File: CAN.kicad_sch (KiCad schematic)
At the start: 15 parts, among them U17 ADM3055E, U18 CDSOT23-T24CAN

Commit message: added more part numbers
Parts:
- R34: P/N (none) -> CRCW08050000Z0EAC
- R35: P/N (none) -> CRCW080559R0FKEA
- U17: Mouser Part Number (none) -> 584-ADM3055EBRIZ; P/N (none) -> ADM3055EBRIZ
- U18: Mouser Part Number (none) -> 652-CDSOT23-T24CAN
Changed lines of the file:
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@@
       (effects (font (size 1.27 1.27)) hide)
     )
-    (property "Datasheet" "" (at 204.47 83.82 0)
+    (property "Datasheet" "https://www.vishay.com/docs/20035/dcrcwe3.pdf" (at 204.47 83.82 0)
       (effects (font (size 1.27 1.27)) hide)
     )
     (property "Mouser Part Number" "71-CRCW080559R0FKEA" (at 204.47 83.82 0)
+      (effects (font (size 1.27 1.27)) hide)
+    )
+    (property "P/N" "CRCW080559R0FKEA" (at 204.47 83.82 0)
       (effects (font (size 1.27 1.27)) hide)
     )
@@
     (property "Datasheet" "https://www.mouser.com/datasheet/2/609/ADM3055E-3057E-1509677.pdf" (at 111.76 82.55 0)
       (effects (font (size 1.524 1.524)) hide)
+    )
+    (property "Mouser Part Number" "584-ADM3055EBRIZ" (at 111.76 85.09 0)
+      (effects (font (size 1.27 1.27)) hide)
+    )
+    (property "P/N" "ADM3055EBRIZ" (at 111.76 85.09 0)
+      (effects (font (size 1.27 1.27)) hide)
     )
     (pin "1")
@@
       (effects (font (size 1.524 1.524)) hide)
     )
-    (property "Mouser Part Number" "" (at 207.01 66.04 0)
+    (property "Mouser Part Number" "652-CDSOT23-T24CAN" (at 207.01 66.04 0)
       (effects (font (size 1.27 1.27)) hide)
     )
@@
       (effects (font (size 1.27 1.27)) hide)
     )
-    (property "Datasheet" "" (at 142.24 99.06 0)
+    (property "Datasheet" "https://www.vishay.com/docs/28773/crcwce3.pdf" (at 142.24 99.06 0)
       (effects (font (size 1.27 1.27)) hide)
     )
@@
       (effects (font (size 1.27 1.27)) hide)
     )
+    (property "P/N" "CRCW08050000Z0EAC" (at 142.24 99.06 0)
+      (effects (font (size 1.27 1.27)) hide)
+    )

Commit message: added part numbers
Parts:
- C33, C38: P/N (none) -> 0805YC106KAT2A
- C34, C35, C39: Mouser Part Number 80-C0805C104K3R -> 80-C0805C104M5R; P/N (none) -> C0805C104M5RACTU
- C36: Mouser Part Number 80-C0805X103K1R3316 -> 80-C0805C104M5R; P/N (none) -> C0805C104M5RACTU
- C37: Mouser Part Number 80-C0805C224J1RECTU -> 80-C0805C224K5R; P/N (none) -> C0805C224K5RACTU
- C40: Mouser Part Number 80-C0805X103K1R3316 -> 80-C0805C103J5R; P/N (none) -> C0805C103J5RACTU
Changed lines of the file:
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@@
       (effects (font (size 1.27 1.27)) hide)
     )
-    (property "Datasheet" "~" (at 74.93 78.74 0)
-      (effects (font (size 1.27 1.27)) hide)
-    )
-    (property "Mouser Part Number" "80-C0805X103K1R3316 " (at 74.93 78.74 0)
+    (property "Datasheet" "https://www.mouser.com/datasheet/2/212/KEM_C1002_X7R_SMD-1102033.pdf" (at 74.93 78.74 0)
+      (effects (font (size 1.27 1.27)) hide)
+    )
+    (property "Mouser Part Number" "80-C0805C104M5R" (at 74.93 78.74 0)
+      (effects (font (size 1.27 1.27)) hide)
+    )
+    (property "P/N" "C0805C104M5RACTU" (at 74.93 78.74 0)
       (effects (font (size 1.27 1.27)) hide)
     )
@@
       (effects (font (size 1.27 1.27)) hide)
     )
-    (property "Datasheet" "~" (at 175.26 74.93 0)
-      (effects (font (size 1.27 1.27)) hide)
-    )
-    (property "Mouser Part Number" "80-C0805X103K1R3316 " (at 175.26 74.93 0)
+    (property "Datasheet" "https://www.mouser.com/datasheet/2/212/KEM_C1002_X7R_SMD-1102033.pdf" (at 175.26 74.93 0)
+      (effects (font (size 1.27 1.27)) hide)
+    )
+    (property "Mouser Part Number" "80-C0805C103J5R" (at 175.26 74.93 0)
+      (effects (font (size 1.27 1.27)) hide)
+    )
+    (property "P/N" "C0805C103J5RACTU" (at 175.26 74.93 0)
       (effects (font (size 1.27 1.27)) hide)
     )
@@
       (effects (font (size 1.27 1.27)) hide)
     )
-    (property "Datasheet" "~" (at 57.785 78.74 0)
-      (effects (font (size 1.27 1.27)) hide)
-    )
-    (property "Mouser Part Number" "80-C0805C104K3R " (at 57.785 78.74 0)
+    (property "Datasheet" "https://www.mouser.com/datasheet/2/212/KEM_C1002_X7R_SMD-1102033.pdf" (at 57.785 78.74 0)
+      (effects (font (size 1.27 1.27)) hide)
+    )
+    (property "Mouser Part Number" "80-C0805C104M5R" (at 57.785 78.74 0)
+      (effects (font (size 1.27 1.27)) hide)
+    )
+    (property "P/N" "C0805C104M5RACTU" (at 57.785 78.74 0)
       (effects (font (size 1.27 1.27)) hide)
     )
@@
       (effects (font (size 1.27 1.27)) hide)
     )
-    (property "Datasheet" "~" (at 167.64 74.93 0)
-      (effects (font (size 1.27 1.27)) hide)
-    )
-    (property "Mouser Part Number" "80-C0805C104K3R " (at 167.64 74.93 0)
+    (property "Datasheet" "https://www.mouser.com/datasheet/2/212/KEM_C1002_X7R_SMD-1102033.pdf" (at 167.64 74.93 0)
+      (effects (font (size 1.27 1.27)) hide)
+    )
+    (property "Mouser Part Number" "80-C0805C104M5R" (at 167.64 74.93 0)
+      (effects (font (size 1.27 1.27)) hide)
+    )
+    (property "P/N" "C0805C104M5RACTU" (at 167.64 74.93 0)
       (effects (font (size 1.27 1.27)) hide)
     )
@@
       (effects (font (size 1.27 1.27)) hide)
     )
-    (property "Datasheet" "" (at 147.32 74.93 0)
-      (effects (font (size 1.27 1.27)) hide)
-    )
-    (property "Mouser Part Number" "80-C0805C224J1RECTU " (at 147.32 74.93 0)
+    (property "Datasheet" "https://www.mouser.com/datasheet/2/212/KEM_C1002_X7R_SMD-1102033.pdf" (at 147.32 74.93 0)
+      (effects (font (size 1.27 1.27)) hide)
+    )
+    (property "Mouser Part Number" "80-C0805C224K5R" (at 147.32 74.93 0)
+      (effects (font (size 1.27 1.27)) hide)
+    )
+    (property "P/N" "C0805C224K5RACTU" (at 147.32 74.93 0)
       (effects (font (size 1.27 1.27)) hide)
     )
@@
       (effects (font (size 1.27 1.27)) hide)
     )
-    (property "Datasheet" "~" (at 69.215 78.74 0)
-      (effects (font (size 1.27 1.27)) hide)
-    )
-    (property "Mouser Part Number" "80-C0805C104K3R " (at 69.215 78.74 0)
+    (property "Datasheet" "https://www.mouser.com/datasheet/2/212/KEM_C1002_X7R_SMD-1102033.pdf" (at 69.215 78.74 0)
+      (effects (font (size 1.27 1.27)) hide)
+    )
+    (property "Mouser Part Number" "80-C0805C104M5R" (at 69.215 78.74 0)
+      (effects (font (size 1.27 1.27)) hide)
+    )
+    (property "P/N" "C0805C104M5RACTU" (at 69.215 78.74 0)
       (effects (font (size 1.27 1.27)) hide)
     )
@@
     )
     (property "Mouser Part Number" "80-C0805C106K8RAUTO " (at 157.48 74.93 0)
+      (effects (font (size 1.27 1.27)) hide)
+    )
+    (property "P/N" "0805YC106KAT2A" (at 157.48 74.93 0)
       (effects (font (size 1.27 1.27)) hide)
     )
@@
       (effects (font (size 1.27 1.27)) hide)
     )
+    (property "P/N" "0805YC106KAT2A" (at 48.895 78.74 0)
+      (effects (font (size 1.27 1.27)) hide)
+    )

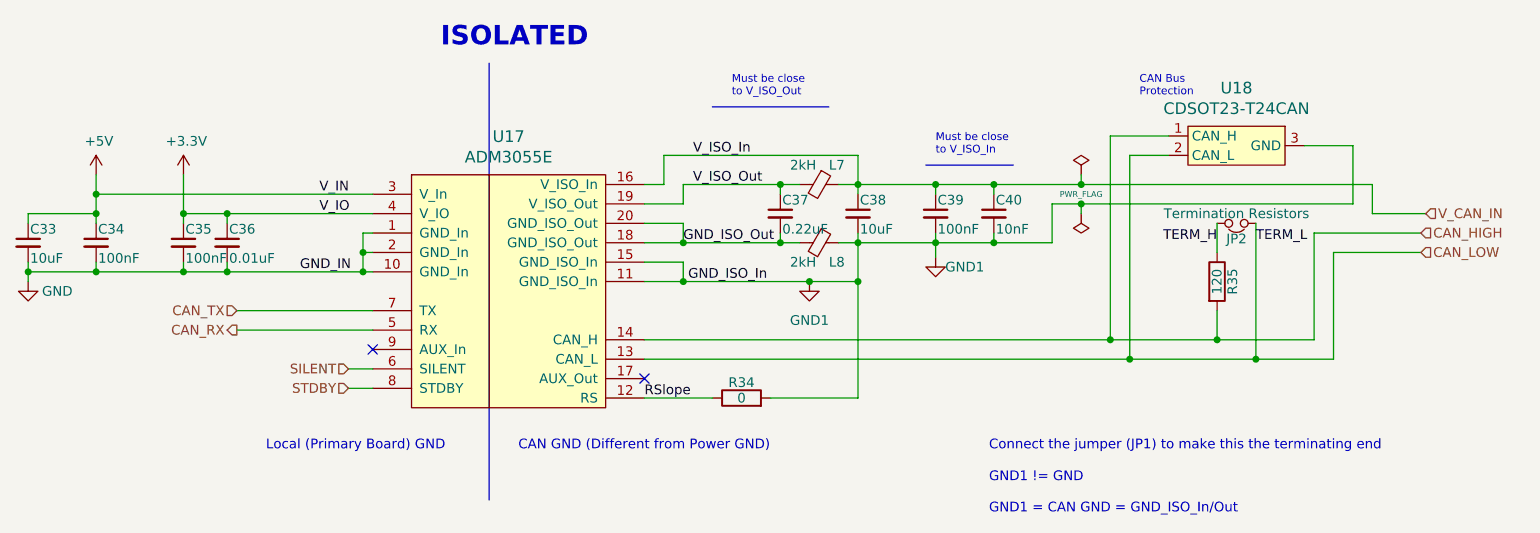
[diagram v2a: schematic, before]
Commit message: v1.2 initial changes
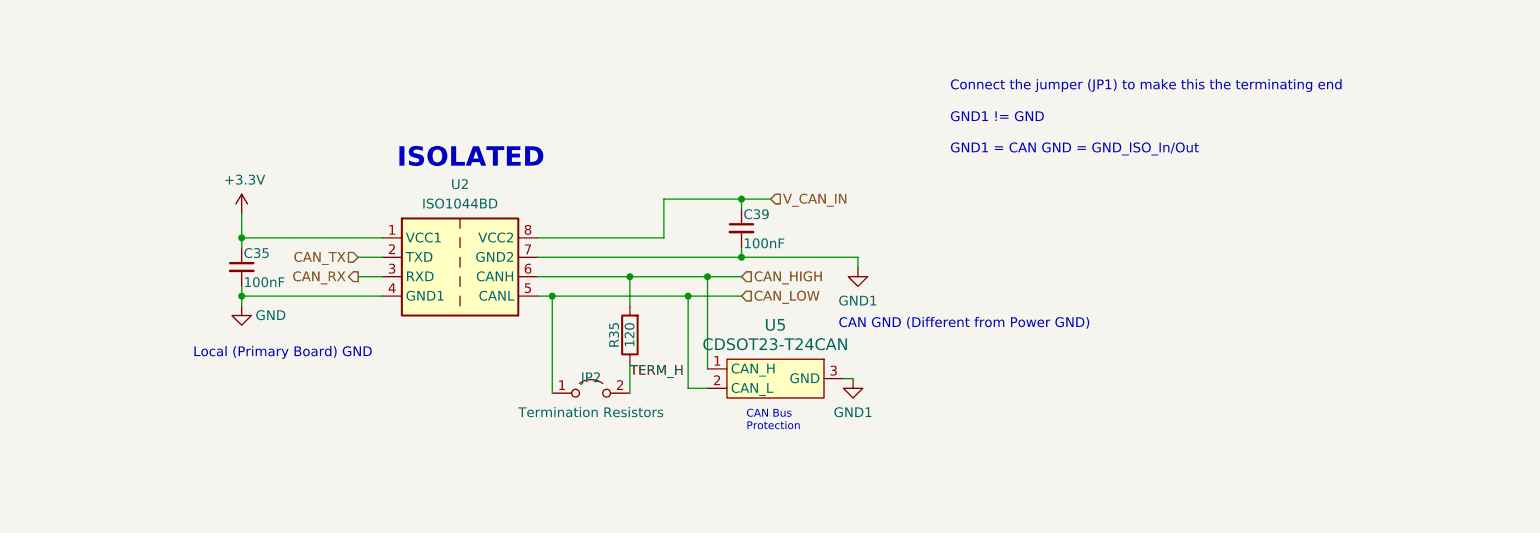
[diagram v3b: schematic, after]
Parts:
- removed C33, C38: 10uF, Capacitor_SMD:C_0805_2012Metric, symbol Device:C_Small
- removed C34: 100nF, Capacitor_SMD:C_0805_2012Metric, symbol Device:C_Small
- removed C36: 0.01uF, Capacitor_SMD:C_0805_2012Metric, symbol Device:C_Small
- removed C37: 0.22uF, Capacitor_SMD:C_0805_2012Metric, symbol Device:C_Small
- removed C40: 10nF, Capacitor_SMD:C_0805_2012Metric, symbol Device:C_Small
- removed JP2: Termination Resistors, Connector_PinHeader_2.54mm:PinHeader_1x02_P2.54mm_Vertical, symbol Device:Jumper_NC_Small
- removed L7, L8: 2kH, Inductor_SMD:L_0805_2012Metric, symbol Device:Ferrite_Bead_Small
- removed R34: 0, Resistor_SMD:R_0805_2012Metric, symbol Device:R
- removed U17: ADM3055E, UTSVT_ICs:SOIC-20W_7.5x15.4mm_Pitch1.27mm, symbol Dashboard-rescue:ADM3055E-utsvt-chips
- removed U18: CDSOT23-T24CAN, Package_TO_SOT_SMD:SOT-23W, symbol Dashboard-rescue:CDSOT23-T24CAN-utsvt-chips
- added JP2: Termination Resistors, Connector_PinHeader_2.54mm:PinHeader_1x02_P2.54mm_Vertical, symbol Jumper:Jumper_2_Open
- added U2: ISO1044BD, Package_SO:SSOP-8_3.9x5.05mm_P1.27mm, symbol utsvt-chips:ISO1044BD
- added U5: CDSOT23-T24CAN, Package_TO_SOT_SMD:SOT-23W, symbol utsvt-chips:CDSOT23-T24CAN
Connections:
- net +3.3V: now also U2.1 (VCC1)
- net CAN_HIGH: now also U2.6 (CANH), U5.1 (CAN_H)
- net CAN_LOW: now also JP2.1 (A), U2.5 (CANL), U5.2 (CAN_L)
- net CAN_RX: now also U2.3 (RXD)
- net CAN_TX: now also U2.2 (TXD)
- net GND: now also U2.4 (GND1)
- net GND1: now also U2.7 (GND2), U5.3 (GND)
- net TERM_H: now also JP2.2 (B)
- net V_CAN_IN: now also U2.8 (VCC2)
- no-connect marks 2 -> 0
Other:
- note removed: "Must be close to V_ISO_In"
- note removed: "Must be close to V_ISO_Out"
